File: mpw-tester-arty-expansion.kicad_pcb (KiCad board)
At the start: 4 copper layers, 53.3 x 61.5 mm, 145 parts, among them J1 USB4105-GF-A, J10 61300211121, J11 61300211121, J12 61300211121, J14 61300311121, J15 61300311121, J18 61300411121, J19 61300711121, J20 61300411121, J3 arty_chipKIT_connector, J4 61300211121, J5 61300311121, J6 61300211121, J7 61300211121, J8 61300211121, J9 61300211121, M1 Arty_A7, Q1 DTC014TEBTL, SW1 JS202011JCQN, SW2 JS202011JCQN, SW3 JS202011JCQN, U1 SN74LVC1G125DCKR, U10 TPD4E02B04DQA, U2 FT232HQ, U3 SN74LVC1G125DCKR, U4 MAX811REUS+T, U5 NTS0102DP, U6 MCP4661-103E/ML, U7 Caravel_breakout_PCB, U8 W25Q32FVSS, U9 MIC2211-AAYML-TR, Y1 ABM8G-12.000MHZ-18-D2Y-T, Y2 ECS-2520MVLC-100-BN-TR

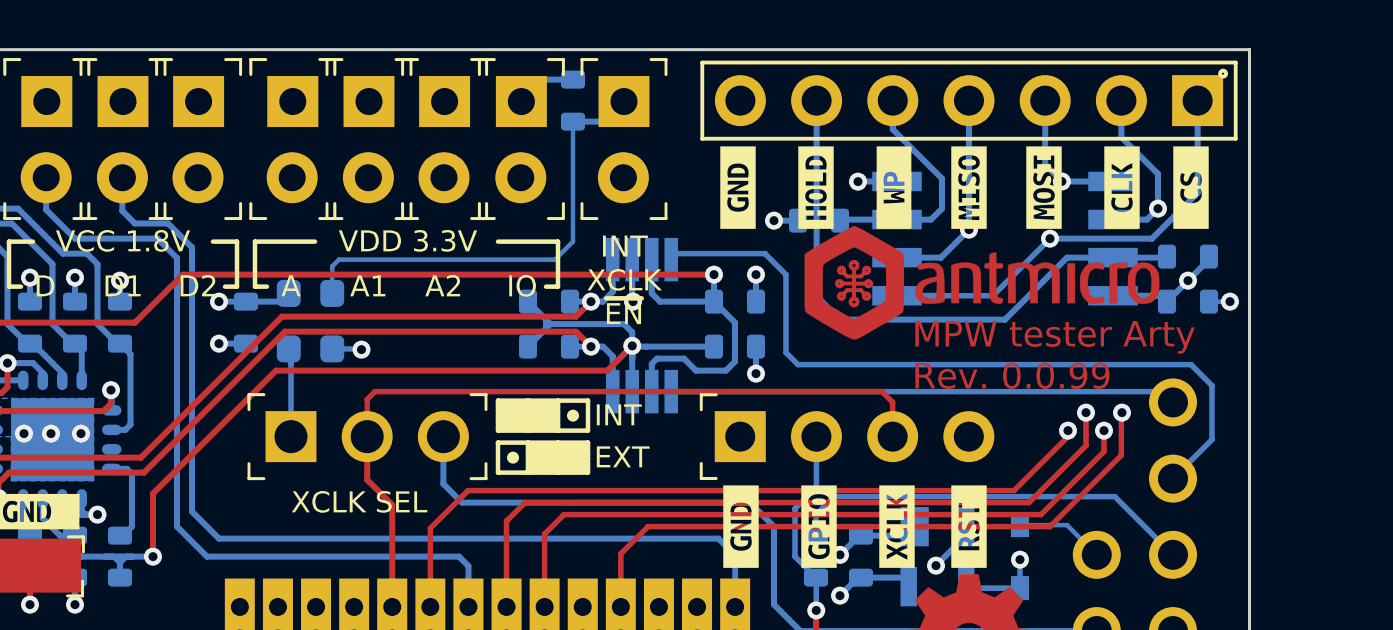
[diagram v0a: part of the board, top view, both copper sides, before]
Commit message: Update PCB name, bump revision to 1.0.0
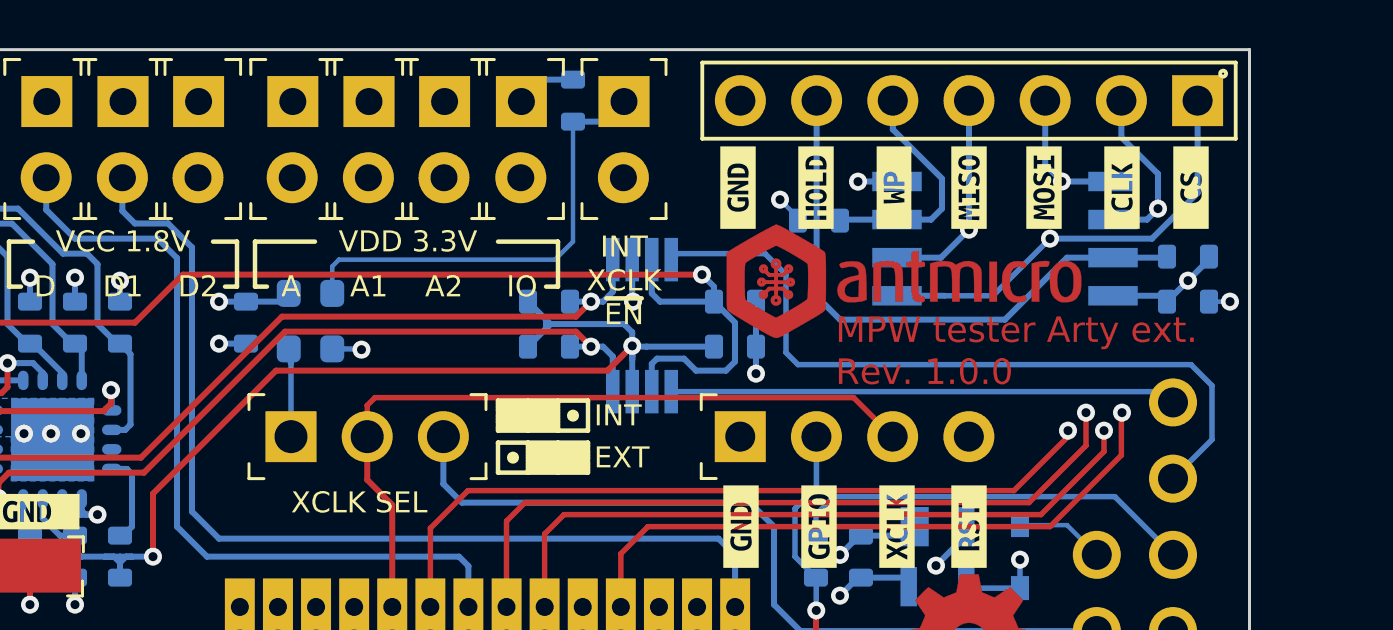
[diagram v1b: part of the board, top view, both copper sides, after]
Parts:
- moved G*** 2.60 mm to (164.8, 73.8) (x2)
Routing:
- net /CRVL_XCLK: track 27.7 -> 26.8 mm
- net AGND: track 130.1 -> 130.7 mm, vias 61 -> 60
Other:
- board text added: "MPW tester Arty ext."
- board text added: "Rev. 1.0.0"
- board text removed: "MPW tester Arty"
- board text removed: "Rev. 0.0.99"
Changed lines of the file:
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@@
   (title_block
     (title "MPW tester Arty expansion")
-    (date "2022-12-02")
-    (rev "0.0.99")
+    (date "2022-12-12")
+    (rev "1.0.0")
   )
   (layers
@@
   )
   (footprint "antmicro-footprints:antmicro-logo_scaled_12mm_mask" (layer "F.Cu")
-    (at 167.4 73.8)
+    (at 164.8 73.75)
     (attr board_only exclude_from_pos_files exclude_from_bom)
     (fp_text reference "G***" (at 0.6096 -2.0955) (layer "F.SilkS") hide
@@
   )
   (footprint "antmicro-footprints:antmicro-logo_scaled_12mm" (layer "F.Cu")
-    (at 167.4 73.8)
+    (at 164.8 73.75)
     (attr board_only exclude_from_pos_files exclude_from_bom)
     (fp_text reference "G***" (at 0.6096 -2.0955) (layer "F.SilkS") hide
@@
   (gr_line (start 128.1 127.55) (end 125.55 125) (layer "Edge.Cuts") (width 0.1))
   (gr_line (start 174.8 125) (end 163.4 125) (layer "Edge.Cuts") (width 0.1))
-  (gr_text "Rev. 0.0.99" (at 165.1 76.9) (layer "F.Cu")
+  (gr_text "Rev. 1.0.0" (at 162.55 76.75) (layer "F.Cu")
     (effects (font (size 0.85 0.85) (thickness 0.18)) (justify left))
   )
-  (gr_text "MPW tester Arty" (at 165.1 75.5) (layer "F.Cu")
+  (gr_text "MPW tester Arty ext." (at 162.55 75.35) (layer "F.Cu")
     (effects (font (size 0.85 0.85) (thickness 0.18)) (justify left))
   )
@@
     (effects (font (size 0.7 0.7) (thickness 0.15)))
   )
-  (gr_text "Rev. 0.0.99" (at 165.1 76.9) (layer "F.Mask")
+  (gr_text "Rev. 1.0.0" (at 162.55 76.75) (layer "F.Mask")
     (effects (font (size 0.85 0.85) (thickness 0.18)) (justify left))
   )
-  (gr_text "MPW tester Arty" (at 165.1 75.5) (layer "F.Mask")
+  (gr_text "MPW tester Arty ext." (at 162.55 75.35) (layer "F.Mask")
     (effects (font (size 0.85 0.85) (thickness 0.18)) (justify left))
   )
@@
   (via (at 135.7 84.5) (size 0.6) (drill 0.3) (layers "F.Cu" "B.Cu") (net 1))
   (via (at 135.5 78.8) (size 0.6) (drill 0.3) (layers "F.Cu" "B.Cu") (net 1))
-  (via (at 159.9 73.5) (size 0.6) (drill 0.3) (layers "F.Cu" "B.Cu") (net 1))
   (via (at 129.7 84.4) (size 0.6) (drill 0.3) (layers "F.Cu" "B.Cu") (net 1))
   (via (at 134.2 73.6) (size 0.6) (drill 0.3) (layers "F.Cu" "B.Cu") (net 1))
@@
   (segment (start 139.15 109.55) (end 139.2 109.5) (width 0.2) (layer "B.Cu") (net 1))
   (segment (start 130.2 105) (end 130.2 106.43) (width 0.2) (layer "B.Cu") (net 1))
-  (segment (start 159.9 74.4) (end 159.9 73.5) (width 0.2) (layer "B.Cu") (net 1))
   (segment (start 136.65 115.15) (end 136.9 114.9) (width 0.2) (layer "B.Cu") (net 1))
   (segment (start 136.9 125.7) (end 136.9 126.6) (width 0.2) (layer "B.Cu") (net 1))
@@
   (segment (start 163.4 82.2) (end 163.3405 82.2) (width 0.2) (layer "B.Cu") (net 1))
   (segment (start 143.75 89.468) (end 143.75 90.368) (width 0.2) (layer "B.Cu") (net 1))
+  (segment (start 159.9 74.4) (end 159.9 75.9) (width 0.2) (layer "B.Cu") (net 1))
   (segment (start 135.7 83.6) (end 135.7 84.5) (width 0.2) (layer "B.Cu") (net 1))
   (segment (start 146.3 107.2) (end 147 107.75) (width 0.2) (layer "B.Cu") (net 1))
@@
   (segment (start 133.6 123.3) (end 133.6 124.5) (width 0.2) (layer "B.Cu") (net 3))
   (segment (start 123.9 103.9) (end 124.4 103.4) (width 0.2) (layer "B.Cu") (net 3))
-  (segment (start 128.9 75.6) (end 128.9 85.7) (width 0.2) (layer "F.Cu") (net 4))
+  (segment (start 129.4 75.1) (end 128.9 75.6) (width 0.2) (layer "F.Cu") (net 4))
+  (segment (start 158.1 73.5) (end 140.8 73.5) (width 0.2) (layer "F.Cu") (net 4))
   (segment (start 140.8 73.5) (end 139.2 75.1) (width 0.2) (layer "F.Cu") (net 4))
   (segment (start 139.2 75.1) (end 129.4 75.1) (width 0.2) (layer "F.Cu") (net 4))
-  (segment (start 129.4 75.1) (end 128.9 75.6) (width 0.2) (layer "F.Cu") (net 4))
-  (segment (start 158.5 73.5) (end 140.8 73.5) (width 0.2) (layer "F.Cu") (net 4))
+  (segment (start 128.9 75.6) (end 128.9 85.7) (width 0.2) (layer "F.Cu") (net 4))
   (via (at 128.9 85.7) (size 0.6) (drill 0.3) (layers "F.Cu" "B.Cu") (net 4))
-  (via (at 158.5 73.5) (size 0.6) (drill 0.3) (layers "F.Cu" "B.Cu") (net 4))
+  (via (at 158.1 73.5) (size 0.6) (drill 0.3) (layers "F.Cu" "B.Cu") (net 4))
   (segment (start 125.54 94.52) (end 127.98 94.52) (width 0.2) (layer "B.Cu") (net 4))
   (segment (start 127.3 93.7) (end 127.3 86.2) (width 0.2) (layer "B.Cu") (net 4))
@@
   (segment (start 158.9 76.7) (end 157.9 76.7) (width 0.2) (layer "B.Cu") (net 4))
   (segment (start 127.8 85.7) (end 128.9 85.7) (width 0.2) (layer "B.Cu") (net 4))
+  (segment (start 158.5 74.4) (end 158.5 73.9) (width 0.2) (layer "B.Cu") (net 4))
   (segment (start 157.5 76.3) (end 156.6 76.3) (width 0.2) (layer "B.Cu") (net 4))
   (segment (start 128 94.5) (end 128 94.4) (width 0.2) (layer "B.Cu") (net 4))
+  (segment (start 158.5 73.9) (end 158.1 73.5) (width 0.2) (layer "B.Cu") (net 4))
   (segment (start 156.425 74.125) (end 156.7 74.4) (width 0.2) (layer "B.Cu") (net 4))
   (segment (start 128 94.4) (end 127.3 93.7) (width 0.2) (layer "B.Cu") (net 4))
   (segment (start 159.2 76.4) (end 158.9 76.7) (width 0.2) (layer "B.Cu") (net 4))
-  (segment (start 158.5 74.4) (end 158.5 73.5) (width 0.2) (layer "B.Cu") (net 4))
   (segment (start 156.6 76.3) (end 156.425 76.475) (width 0.2) (layer "B.Cu") (net 4))
   (segment (start 127.98 94.52) (end 128 94.5) (width 0.2) (layer "B.Cu") (net 4))
@@
   (via (at 146.95 90.368) (size 0.6) (drill 0.3) (layers "F.Cu" "B.Cu") (net 8))
   (via (at 162.7 84.2) (size 0.6) (drill 0.3) (layers "F.Cu" "B.Cu") (net 8))
-  (via (at 160.5 71.7) (size 0.6) (drill 0.3) (layers "F.Cu" "B.Cu") (net 8))
   (via (at 142 74.4) (size 0.6) (drill 0.3) (layers "F.Cu" "B.Cu") (net 8))
   (via (at 151.75 90.368) (size 0.6) (drill 0.3) (layers "F.Cu" "B.Cu") (net 8))
   (via (at 133.2 76.75) (size 0.6) (drill 0.3) (layers "F.Cu" "B.Cu") (net 8))
+  (via (at 160.7 71) (size 0.6) (drill 0.3) (layers "F.Cu" "B.Cu") (net 8))
   (via (at 153.35 90.368) (size 0.6) (drill 0.3) (layers "F.Cu" "B.Cu") (net 8))
   (segment (start 151.25 108.6) (end 152.3 108.6) (width 0.2) (layer "B.Cu") (net 8))
@@
   (segment (start 153.8 67) (end 152.81 67) (width 0.2) (layer "B.Cu") (net 8))
   (segment (start 171.8 74.205) (end 173.405 74.205) (width 0.2) (layer "B.Cu") (net 8))
+  (segment (start 161.3 71.7) (end 161.3 71.6) (width 0.15) (layer "B.Cu") (net 8))
   (segment (start 148.55 89.468) (end 148.55 90.368) (width 0.2) (layer "B.Cu") (net 8))
   (segment (start 155.25 108.6) (end 155.25 108.15) (width 0.2) (layer "B.Cu") (net 8))
@@
   (segment (start 155.5 107.9) (end 156.2 107.9) (width 0.2) (layer "B.Cu") (net 8))
   (segment (start 142.9 74.4) (end 142 74.4) (width 0.2) (layer "B.Cu") (net 8))
-  (segment (start 161.3 71.7) (end 160.5 71.7) (width 0.2) (layer "B.Cu") (net 8))
+  (segment (start 161.3 71.6) (end 160.7 71) (width 0.15) (layer "B.Cu") (net 8))
   (segment (start 175 73) (end 174.3 73.7) (width 0.2) (layer "B.Cu") (net 8))
   (segment (start 163.3 83.6) (end 162.7 84.2) (width 0.2) (layer "B.Cu") (net 8))
@@
   (segment (start 147.775 84.578) (end 147.775 81.175) (width 0.2) (layer "F.Cu") (net 51))
   (segment (start 147.775 84.578) (end 147.775 86.128) (width 0.2) (layer "F.Cu") (net 51))
-  (segment (start 147.2 77.4) (end 164.1 77.4) (width 0.182) (layer "F.Cu") (net 51))
-  (segment (start 164.455 77.755) (end 164.455 78.9) (width 0.182) (layer "F.Cu") (net 51))
+  (segment (start 163.155 77.6) (end 147.2 77.6) (width 0.182) (layer "F.Cu") (net 51))
+  (segment (start 147.2 77.6) (end 146.94 77.86) (width 0.182) (layer "F.Cu") (net 51))
   (segment (start 146.94 80.34) (end 147.775 81.175) (width 0.2) (layer "F.Cu") (net 51))
-  (segment (start 164.1 77.4) (end 164.455 77.755) (width 0.182) (layer "F.Cu") (net 51))
-  (segment (start 146.94 78.9) (end 146.94 77.66) (width 0.182) (layer "F.Cu") (net 51))
-  (segment (start 146.94 77.66) (end 147.2 77.4) (width 0.182) (layer "F.Cu") (net 51))
+  (segment (start 146.94 77.86) (end 146.94 78.9) (width 0.182) (layer "F.Cu") (net 51))
+  (segment (start 164.455 78.9) (end 163.155 77.6) (width 0.182) (layer "F.Cu") (net 51))
   (segment (start 144.375 76.425) (end 144.4 76.45) (width 0.182) (layer "B.Cu") (net 52))
   (segment (start 144.4 76.45) (end 144.4 78.9) (width 0.182) (layer "B.Cu") (net 52))
